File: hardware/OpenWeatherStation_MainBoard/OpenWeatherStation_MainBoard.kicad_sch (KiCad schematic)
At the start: 0 parts

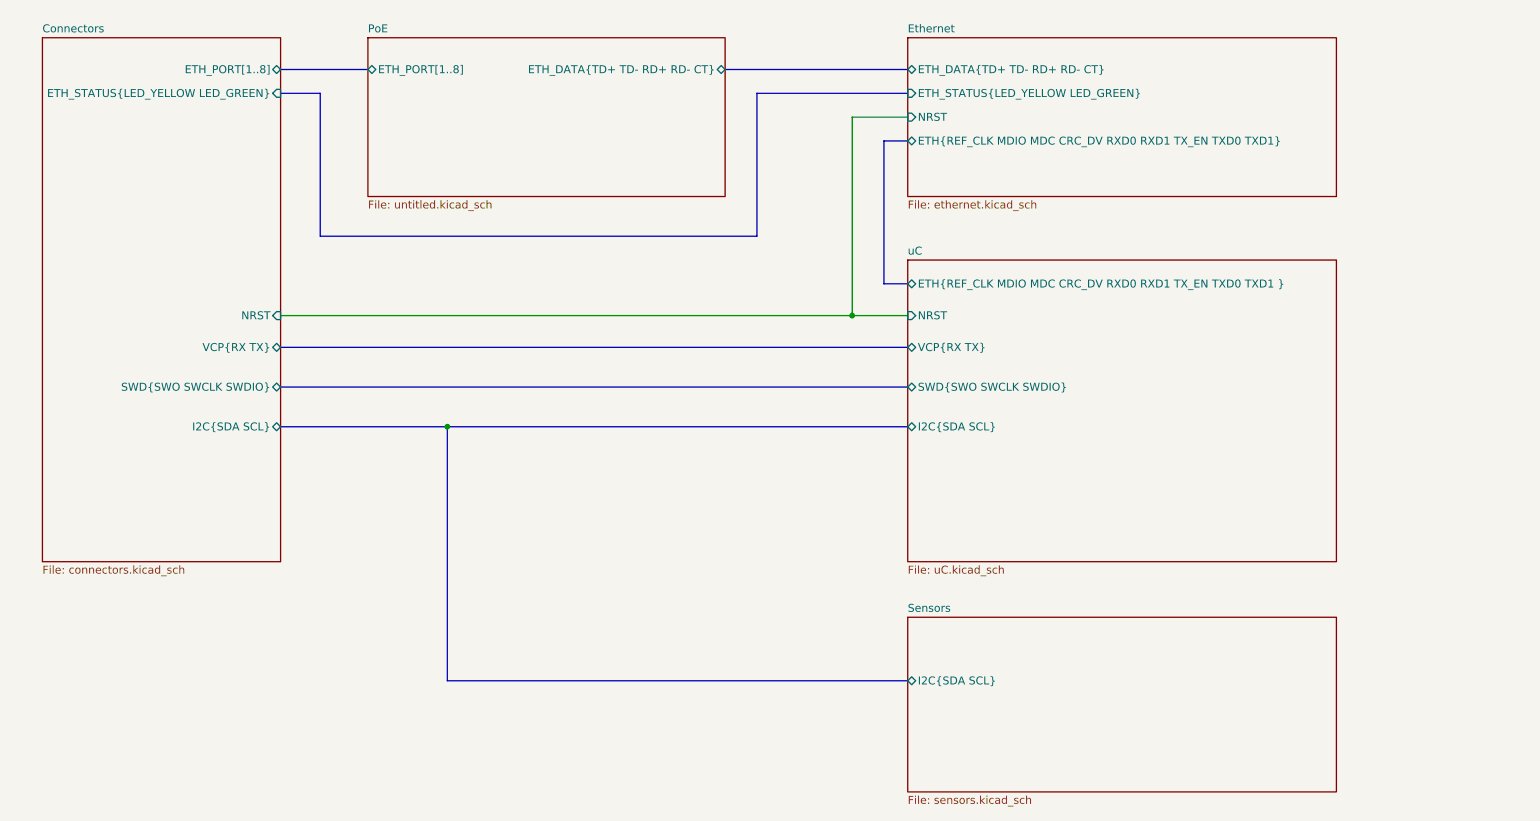
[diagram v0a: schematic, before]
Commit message: poe wip
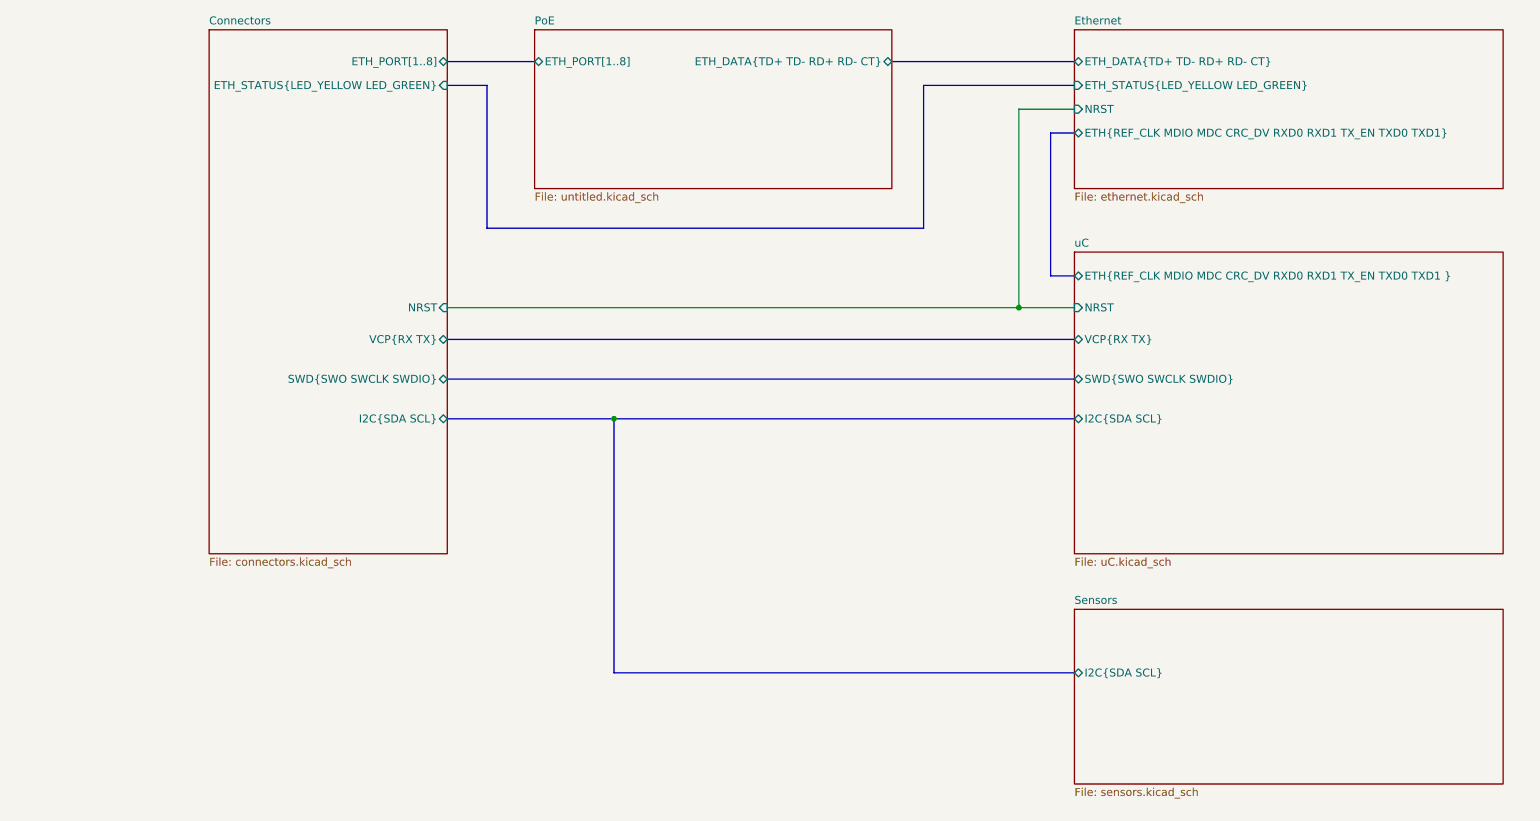
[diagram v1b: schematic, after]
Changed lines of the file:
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@@
 (kicad_sch (version 20230121) (generator eeschema)
   (paper "A4")
-  (junction (at 81.28 93.98) (diameter 0) (color 0 0 0 0)
+  (junction (at 107.95 92.71) (diameter 0) (color 0 0 0 0)
   )
-  (junction (at 146.05 76.2) (diameter 0) (color 0 0 0 0)
+  (junction (at 172.72 74.93) (diameter 0) (color 0 0 0 0)
   )
-  (bus (pts (xy 60.96 63.5) (xy 130.81 63.5))
+  (bus (pts (xy 87.63 62.23) (xy 157.48 62.23))
     (stroke (width 0) (type default))
   )
-  (bus (pts (xy 81.28 93.98) (xy 81.28 134.62))
+  (bus (pts (xy 107.95 92.71) (xy 107.95 133.35))
     (stroke (width 0) (type default))
   )
-  (bus (pts (xy 151.13 48.26) (xy 151.13 71.12))
+  (bus (pts (xy 177.8 46.99) (xy 177.8 69.85))
     (stroke (width 0) (type default))
   )
-  (wire (pts (xy 146.05 44.45) (xy 146.05 76.2))
+  (wire (pts (xy 172.72 43.18) (xy 172.72 74.93))
     (stroke (width 0) (type default))
   )
-  (wire (pts (xy 154.94 44.45) (xy 146.05 44.45))
+  (wire (pts (xy 181.61 43.18) (xy 172.72 43.18))
     (stroke (width 0) (type default))
   )
-  (wire (pts (xy 54.61 76.2) (xy 146.05 76.2))
+  (wire (pts (xy 81.28 74.93) (xy 172.72 74.93))
     (stroke (width 0) (type default))
   )
-  (bus (pts (xy 54.61 87.63) (xy 154.94 87.63))
+  (bus (pts (xy 81.28 86.36) (xy 181.61 86.36))
     (stroke (width 0) (type default))
   )
-  (bus (pts (xy 154.94 48.26) (xy 151.13 48.26))
+  (bus (pts (xy 181.61 46.99) (xy 177.8 46.99))
     (stroke (width 0) (type default))
   )
-  (bus (pts (xy 54.61 40.64) (xy 60.96 40.64))
+  (bus (pts (xy 81.28 39.37) (xy 87.63 39.37))
     (stroke (width 0) (type default))
   )
-  (bus (pts (xy 151.13 71.12) (xy 154.94 71.12))
+  (bus (pts (xy 177.8 69.85) (xy 181.61 69.85))
     (stroke (width 0) (type default))
   )
-  (wire (pts (xy 146.05 76.2) (xy 154.94 76.2))
+  (wire (pts (xy 172.72 74.93) (xy 181.61 74.93))
     (stroke (width 0) (type default))
   )
-  (bus (pts (xy 81.28 134.62) (xy 154.94 134.62))
+  (bus (pts (xy 107.95 133.35) (xy 181.61 133.35))
     (stroke (width 0) (type default))
   )
-  (bus (pts (xy 54.61 36.83) (xy 68.58 36.83))
+  (bus (pts (xy 81.28 35.56) (xy 95.25 35.56))
     (stroke (width 0) (type default))
   )
-  (bus (pts (xy 130.81 63.5) (xy 130.81 40.64))
+  (bus (pts (xy 157.48 62.23) (xy 157.48 39.37))
     (stroke (width 0) (type default))
   )
-  (bus (pts (xy 130.81 40.64) (xy 154.94 40.64))
+  (bus (pts (xy 157.48 39.37) (xy 181.61 39.37))
     (stroke (width 0) (type default))
   )
-  (bus (pts (xy 154.94 81.28) (xy 54.61 81.28))
+  (bus (pts (xy 181.61 80.01) (xy 81.28 80.01))
     (stroke (width 0) (type default))
   )
-  (bus (pts (xy 60.96 40.64) (xy 60.96 63.5))
+  (bus (pts (xy 87.63 39.37) (xy 87.63 62.23))
     (stroke (width 0) (type default))
   )
-  (bus (pts (xy 54.61 93.98) (xy 81.28 93.98))
+  (bus (pts (xy 81.28 92.71) (xy 107.95 92.71))
     (stroke (width 0) (type default))
   )
-  (bus (pts (xy 154.94 93.98) (xy 81.28 93.98))
+  (bus (pts (xy 181.61 92.71) (xy 107.95 92.71))
     (stroke (width 0) (type default))
   )
-  (bus (pts (xy 125.73 36.83) (xy 154.94 36.83))
+  (bus (pts (xy 152.4 35.56) (xy 181.61 35.56))
     (stroke (width 0) (type default))
   )
-  (sheet (at 154.94 31.75) (size 68.58 25.4) (fields_autoplaced)
+  (sheet (at 181.61 30.48) (size 68.58 25.4) (fields_autoplaced)
     (stroke (width 0.1524) (type solid))
     (fill (color 0 0 0 0.0000))
-    (property "Sheetname" "Ethernet" (at 154.94 31.0384 0)
+    (property "Sheetname" "Ethernet" (at 181.61 29.7684 0)
       (effects (font (size 1.27 1.27)) (justify left bottom))
     )
-    (property "Sheetfile" "ethernet.kicad_sch" (at 154.94 57.7346 0)
+    (property "Sheetfile" "ethernet.kicad_sch" (at 181.61 56.4646 0)
       (effects (font (size 1.27 1.27)) (justify left top))
     )
-    (pin "ETH_STATUS{LED_YELLOW LED_GREEN}" input (at 154.94 40.64 180)
+    (pin "ETH_STATUS{LED_YELLOW LED_GREEN}" input (at 181.61 39.37 180)
       (effects (font (size 1.27 1.27)) (justify left))
     )
-    (pin "ETH_DATA{TD+ TD- RD+ RD- CT}" bidirectional (at 154.94 36.83 180)
+    (pin "ETH_DATA{TD+ TD- RD+ RD- CT}" bidirectional (at 181.61 35.56 180)
       (effects (font (size 1.27 1.27)) (justify left))
     )
-    (pin "ETH{REF_CLK MDIO MDC CRC_DV RXD0 RXD1 TX_EN TXD0 TXD1}" bidirectional (at 154.94 48.26 180)
+    (pin "ETH{REF_CLK MDIO MDC CRC_DV RXD0 RXD1 TX_EN TXD0 TXD1}" bidirectional (at 181.61 46.99 180)
       (effects (font (size 1.27 1.27)) (justify left))
     )
-    (pin "NRST" input (at 154.94 44.45 180)
+    (pin "NRST" input (at 181.61 43.18 180)
       (effects (font (size 1.27 1.27)) (justify left))
     )
@@
     )
   )
-  (sheet (at 16.51 31.75) (size 38.1 83.82) (fields_autoplaced)
+  (sheet (at 43.18 30.48) (size 38.1 83.82) (fields_autoplaced)
     (stroke (width 0.1524) (type solid))
     (fill (color 0 0 0 0.0000))
-    (property "Sheetname" "Connectors" (at 16.51 31.0384 0)
+    (property "Sheetname" "Connectors" (at 43.18 29.7684 0)
       (effects (font (size 1.27 1.27)) (justify left bottom))
     )
-    (property "Sheetfile" "connectors.kicad_sch" (at 16.51 116.1546 0)
+    (property "Sheetfile" "connectors.kicad_sch" (at 43.18 114.8846 0)
       (effects (font (size 1.27 1.27)) (justify left top))
     )
-    (pin "I2C{SDA SCL}" bidirectional (at 54.61 93.98 0)
+    (pin "I2C{SDA SCL}" bidirectional (at 81.28 92.71 0)
       (effects (font (size 1.27 1.27)) (justify right))
     )
-    (pin "ETH_PORT[1..8]" bidirectional (at 54.61 36.83 0)
+    (pin "ETH_PORT[1..8]" bidirectional (at 81.28 35.56 0)
       (effects (font (size 1.27 1.27)) (justify right))
     )
-    (pin "ETH_STATUS{LED_YELLOW LED_GREEN}" input (at 54.61 40.64 0)
+    (pin "ETH_STATUS{LED_YELLOW LED_GREEN}" input (at 81.28 39.37 0)
       (effects (font (size 1.27 1.27)) (justify right))
     )
-    (pin "VCP{RX TX}" bidirectional (at 54.61 81.28 0)
+    (pin "VCP{RX TX}" bidirectional (at 81.28 80.01 0)
       (effects (font (size 1.27 1.27)) (justify right))
     )
-    (pin "NRST" input (at 54.61 76.2 0)
+    (pin "NRST" input (at 81.28 74.93 0)
       (effects (font (size 1.27 1.27)) (justify right))
     )
-    (pin "SWD{SWO SWCLK SWDIO}" bidirectional (at 54.61 87.63 0)
+    (pin "SWD{SWO SWCLK SWDIO}" bidirectional (at 81.28 86.36 0)
       (effects (font (size 1.27 1.27)) (justify right))
     )
@@
     )
   )
-  (sheet (at 68.58 31.75) (size 57.15 25.4) (fields_autoplaced)
+  (sheet (at 95.25 30.48) (size 57.15 25.4) (fields_autoplaced)
     (stroke (width 0.1524) (type solid))
     (fill (color 0 0 0 0.0000))
-    (property "Sheetname" "PoE" (at 68.58 31.0384 0)
+    (property "Sheetname" "PoE" (at 95.25 29.7684 0)
       (effects (font (size 1.27 1.27)) (justify left bottom))
     )
-    (property "Sheetfile" "untitled.kicad_sch" (at 68.58 57.7346 0)
+    (property "Sheetfile" "untitled.kicad_sch" (at 95.25 56.4646 0)
       (effects (font (size 1.27 1.27)) (justify left top))
     )
-    (pin "ETH_PORT[1..8]" bidirectional (at 68.58 36.83 180)
+    (pin "ETH_PORT[1..8]" bidirectional (at 95.25 35.56 180)
       (effects (font (size 1.27 1.27)) (justify left))
     )
-    (pin "ETH_DATA{TD+ TD- RD+ RD- CT}" bidirectional (at 125.73 36.83 0)
+    (pin "ETH_DATA{TD+ TD- RD+ RD- CT}" bidirectional (at 152.4 35.56 0)
       (effects (font (size 1.27 1.27)) (justify right))
     )
@@
     )
   )
-  (sheet (at 154.94 124.46) (size 68.58 27.94) (fields_autoplaced)
+  (sheet (at 181.61 123.19) (size 68.58 27.94) (fields_autoplaced)
     (stroke (width 0.1524) (type solid))
     (fill (color 0 0 0 0.0000))
-    (property "Sheetname" "Sensors" (at 154.94 123.7484 0)
+    (property "Sheetname" "Sensors" (at 181.61 122.4784 0)
       (effects (font (size 1.27 1.27)) (justify left bottom))
     )
-    (property "Sheetfile" "sensors.kicad_sch" (at 154.94 152.9846 0)
+    (property "Sheetfile" "sensors.kicad_sch" (at 181.61 151.7146 0)
       (effects (font (size 1.27 1.27)) (justify left top))
     )
-    (pin "I2C{SDA SCL}" bidirectional (at 154.94 134.62 180)
+    (pin "I2C{SDA SCL}" bidirectional (at 181.61 133.35 180)
       (effects (font (size 1.27 1.27)) (justify left))
     )
@@
     )
   )
-  (sheet (at 154.94 67.31) (size 68.58 48.26) (fields_autoplaced)
+  (sheet (at 181.61 66.04) (size 68.58 48.26) (fields_autoplaced)
     (stroke (width 0.1524) (type solid))
     (fill (color 0 0 0 0.0000))
-    (property "Sheetname" "uC" (at 154.94 66.5984 0)
+    (property "Sheetname" "uC" (at 181.61 65.3284 0)
       (effects (font (size 1.27 1.27)) (justify left bottom))
     )
-    (property "Sheetfile" "uC.kicad_sch" (at 154.94 116.1546 0)
+    (property "Sheetfile" "uC.kicad_sch" (at 181.61 114.8846 0)
       (effects (font (size 1.27 1.27)) (justify left top))
     )
-    (pin "I2C{SDA SCL}" bidirectional (at 154.94 93.98 180)
+    (pin "I2C{SDA SCL}" bidirectional (at 181.61 92.71 180)
       (effects (font (size 1.27 1.27)) (justify left))
     )
-    (pin "ETH{REF_CLK MDIO MDC CRC_DV RXD0 RXD1 TX_EN TXD0 TXD1 }" bidirectional (at 154.94 71.12 180)
+    (pin "ETH{REF_CLK MDIO MDC CRC_DV RXD0 RXD1 TX_EN TXD0 TXD1 }" bidirectional (at 181.61 69.85 180)
       (effects (font (size 1.27 1.27)) (justify left))
     )
-    (pin "VCP{RX TX}" bidirectional (at 154.94 81.28 180)
+    (pin "VCP{RX TX}" bidirectional (at 181.61 80.01 180)
       (effects (font (size 1.27 1.27)) (justify left))
     )
-    (pin "NRST" input (at 154.94 76.2 180)
+    (pin "NRST" input (at 181.61 74.93 180)
       (effects (font (size 1.27 1.27)) (justify left))
     )
-    (pin "SWD{SWO SWCLK SWDIO}" bidirectional (at 154.94 87.63 180)
+    (pin "SWD{SWO SWCLK SWDIO}" bidirectional (at 181.61 86.36 180)
       (effects (font (size 1.27 1.27)) (justify left))
     )

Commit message: electrical design wip
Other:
- company: (none) -> Vital Septfonds
- title: (none) -> Open Wheather Station
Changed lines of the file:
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@@
 (kicad_sch (version 20230121) (generator eeschema)
   (paper "A4")
+  (title_block
+    (title "Open Wheather Station")
+    (date "2024-01-02")
+    (rev "1.0")
+    (company "Vital Septfonds")
+  )
   (junction (at 107.95 92.71) (diameter 0) (color 0 0 0 0)
   )
